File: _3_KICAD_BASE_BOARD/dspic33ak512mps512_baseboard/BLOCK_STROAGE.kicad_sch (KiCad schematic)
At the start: 1 part, among them U3 FM24W256G

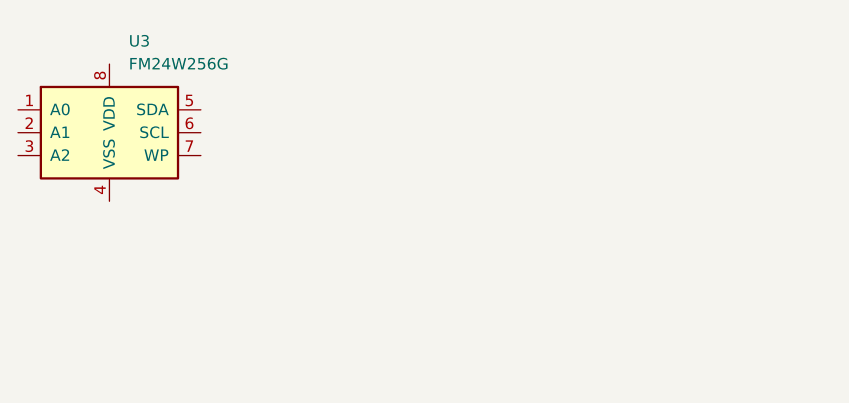
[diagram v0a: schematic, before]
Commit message: feat : 회로 작업중
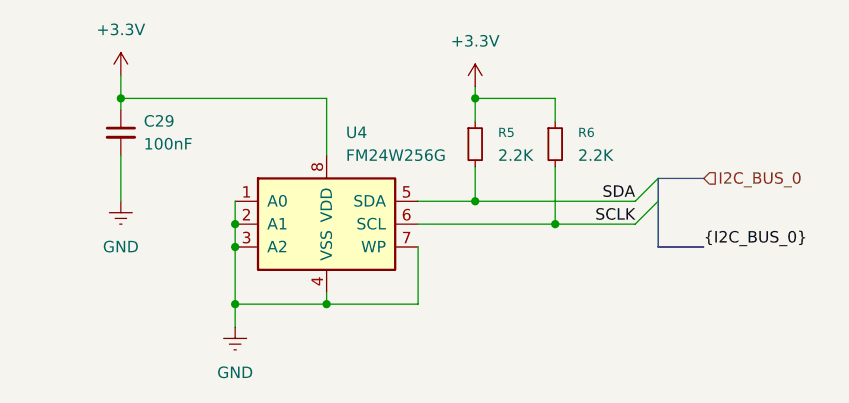
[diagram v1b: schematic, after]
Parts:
- added C29: 100nF, Capacitor_SMD:C_0603_1608Metric, symbol Device:C_Small
- added R5, R6: 2.2K, Resistor_SMD:R_0603_1608Metric, symbol Device:R_Small
- renumbered U3 to U4
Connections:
- net GND: now reaches U4.1 (A0)
- net GND: now also U4.2 (A1), U4.3 (A2), U4.4 (VSS), U4.7 (WP), C29.2
- net SDA: now reaches U4.5 (SDA)
- net SDA: now also R5.2
- net SCLK: now reaches U4.6 (SCL)
- net SCLK: now also R6.2
- net +3.3V: now reaches U4.8 (VDD)
- net +3.3V: now also C29.1, R5.1, R6.1
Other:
- moved on the sheet: U4
